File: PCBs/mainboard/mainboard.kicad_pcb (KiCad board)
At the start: 2 copper layers, 76.6 x 80 mm, 32 parts, among them J1 USB_C_Receptacle_USB2.0_16P, SW1 SW_Push_Dual, SW2 SW_Push_Dual, SW3 SW_Push_Dual, U3 ESP32-S3-WROOM-1

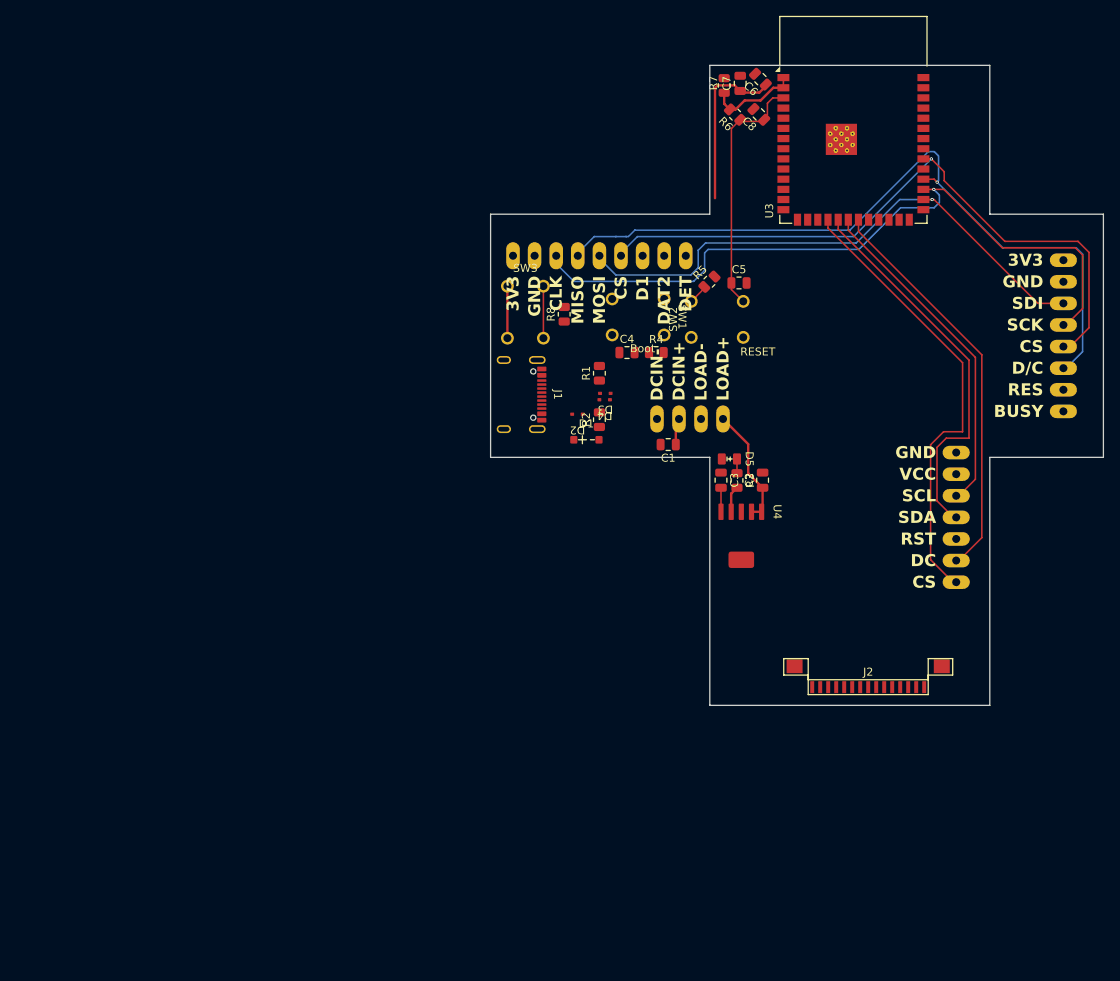
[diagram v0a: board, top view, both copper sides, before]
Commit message: Layouting pt.1
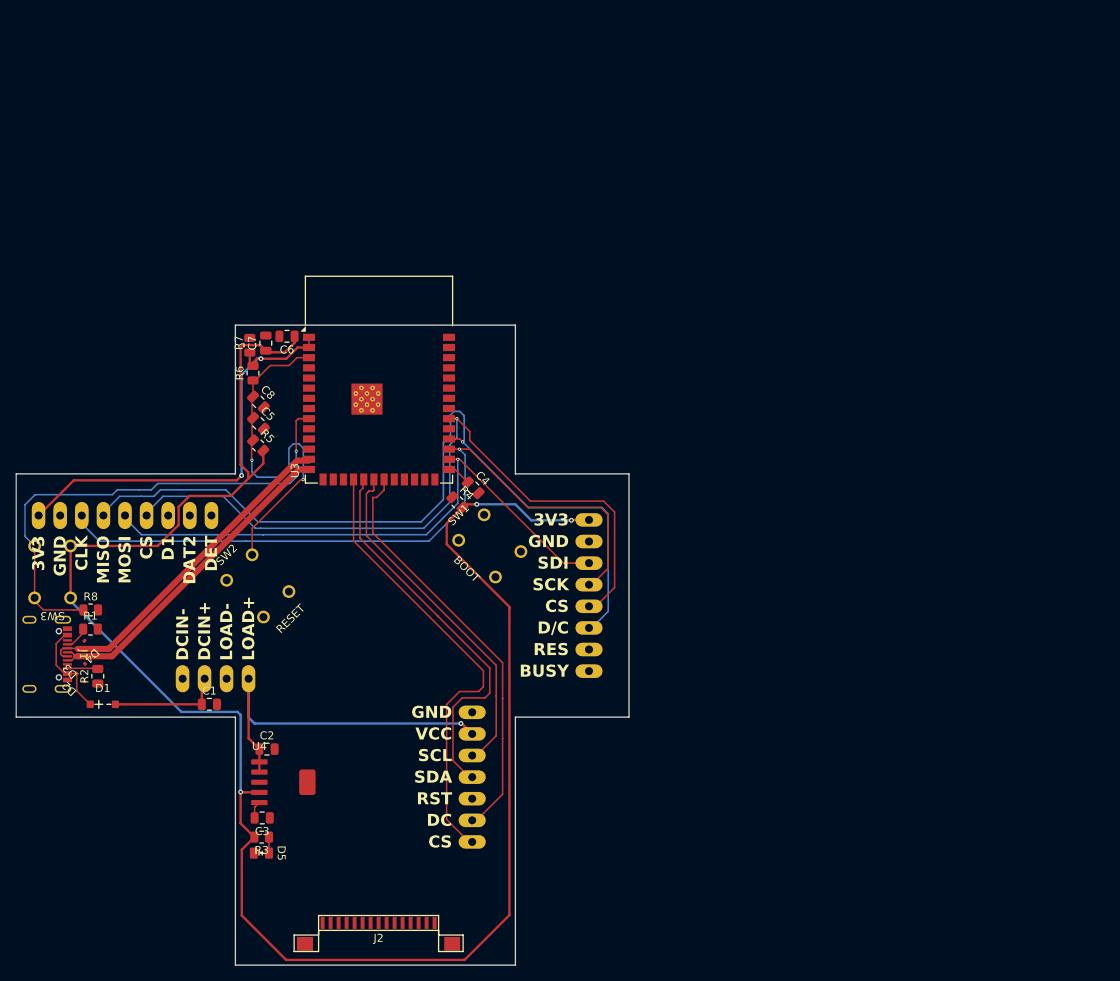
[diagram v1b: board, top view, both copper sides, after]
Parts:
- moved D5 76.5 mm to (83.2, 134.1)
- moved R3 74.3 mm to (83.2, 132.1), turned to 180 degrees
- moved D3 73.5 mm to (60.6, 109.9), turned to 135 degrees
- moved D4 72.3 mm to (60.6, 108.0), turned to -135 degrees
- moved C8 72.1 mm to (82.8, 77.7), turned to -45 degrees
- moved C3 71.2 mm to (83.2, 129.7), turned to 180 degrees
- moved R1 71.2 mm to (61.8, 106.1), turned to 0 degrees
- moved C2 70.5 mm to (83.8, 121.1), turned to 0 degrees
- moved R2 70.4 mm to (62.7, 112.0)
- moved D2 70.3 mm to (60.5, 112.1), turned to 135 degrees
- moved R8 69.8 mm to (61.8, 103.7), turned to 0 degrees
- moved U4 69.1 mm to (82.9, 125.2), turned to 0 degrees
- moved D1 68.9 mm to (63.3, 115.5)
- moved U2 68.7 mm to (109.5, 132.7)
- moved R6 68.4 mm to (82.1, 74.1), turned to 90 degrees
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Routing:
- net VCC_3V3: track 30.8 -> 229.9 mm, vias 0 -> 3
- net GPIO16: track 6.50 -> 63.2 mm, vias 0 -> 1
- net ESP_3V3: track 11.7 -> 54.8 mm, vias 0 -> 2
- net D-: track 0.00 -> 42.2 mm
- net D+: track 0.00 -> 41.3 mm
- net VCC_4V5: track 15.0 -> 45.9 mm, vias 0 -> 1
- net CHIP_PU: track 33.2 -> 46.1 mm, vias 0 -> 2
- net Net-(D1-A): track 0.00 -> 12.0 mm
- net VCC_5V: track 3.37 -> 14.2 mm
- net GPIO37: track 93.5 -> 102.6 mm
- net GPIO39: track 83.8 -> 92.7 mm
- net Net-(J1-CC2): track 0.00 -> 3.83 mm
- net Net-(J1-CC1): track 0.00 -> 3.05 mm
- net GPIO0: track 0.00 -> 3.03 mm
- net GPIO35: track 70.9 -> 72.8 mm
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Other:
- copper layers 2 -> 4
- board text added: "BOOT"
- board text removed: "Boot"
